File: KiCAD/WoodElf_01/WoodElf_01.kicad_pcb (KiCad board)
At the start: 2 copper layers, 97.7 x 102.4 mm, 122 parts, among them T10 BlankThrough-Hole, T11 BlankThrough-Hole, T12 BlankThrough-Hole, T13 BlankThrough-Hole, T2 BlankThrough-Hole, T3 BlankThrough-Hole, T4 BlankThrough-Hole, T5 BlankThrough-Hole, T6 BlankThrough-Hole, T7 BlankThrough-Hole, T8 BlankThrough-Hole, T9 BlankThrough-Hole

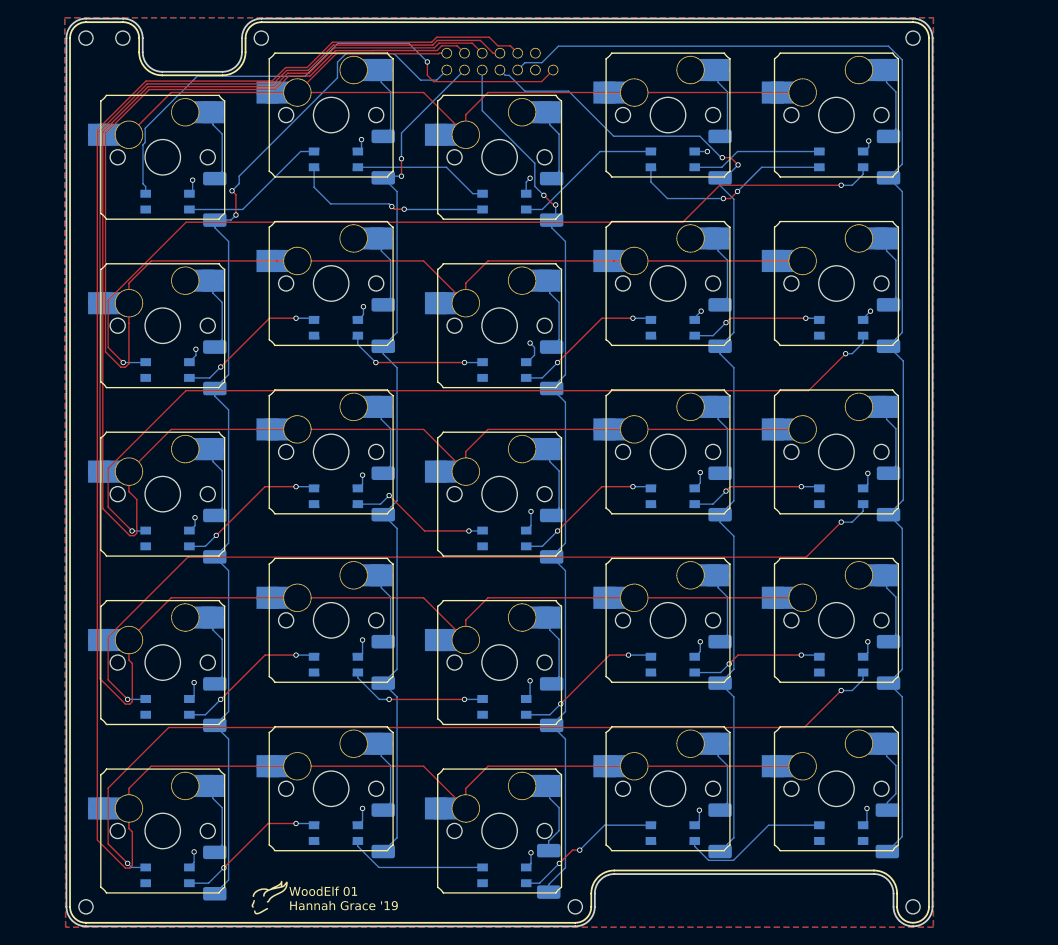
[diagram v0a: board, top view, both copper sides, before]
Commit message: completely redid everything
properly this time.
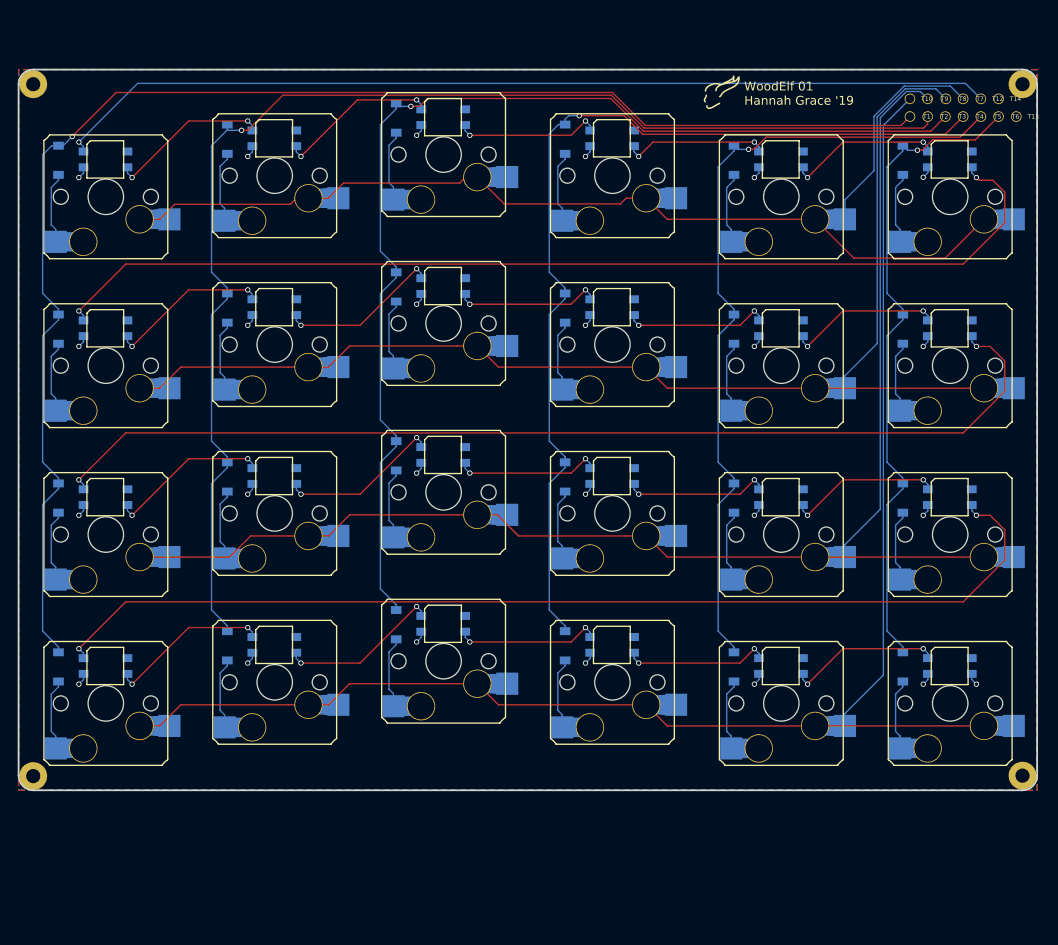
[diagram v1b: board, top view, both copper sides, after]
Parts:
- removed D21, D22, D23, D24, D25: DIODE, Diode_SMD:D_2010_5025Metric_Pad1.52x2.65mm_HandSolder
- removed the G*** at (135.0, 151.5)
- removed the G*** at (121.0, 151.6)
- removed H21, H22, H23, H24, H25: Kailh_HotSwap_SwitchMount, WoodElf_Lib:Kailh_HotSwap_Socket
- removed L21, L22, L23, L24, L25: SK6812MINI, WoodElf_Lib:LED_SK6812MINI_PLCC4_3.5x3.5mm_P1.75mm
- removed the Mount at (120.1, 54.4)
- removed the Mount at (104.5, 54.4)
- removed the Mount at (155.5, 152.4)
- removed the Mount at (193.6, 152.4)
- removed the Mount at (100.3, 152.4)
- removed the Mount at (100.3, 54.4)
- removed the Mount at (193.6, 54.4)
- removed S21, S22, S23, S24, S25: Kailh_RGB_Switch, WoodElf_Lib:SW_Cherry_MX1A_1.00u_PCB
- removed T11, wT1: BlankThrough-Hole, WoodElf_Lib:BlankThrough-Hole
- added D27: DIODE, WoodElf_Lib:D_SOD-123, B.Cu at (192.4, 125.3)
- added D28: DIODE, WoodElf_Lib:D_SOD-123, B.Cu at (192.4, 106.3)
- added D29: DIODE, WoodElf_Lib:D_SOD-123, B.Cu at (192.4, 87.2)
- added D30: DIODE, WoodElf_Lib:D_SOD-123, B.Cu at (192.4, 68.2)
- added G***: Tiefling_Logo, WoodElf_Lib:Tiefling_Logo, B.Cu at (186.3, 60.8)
- added G***: Tiefling_Logo, WoodElf_Lib:Tiefling_Logo, F.Cu at (172.0, 60.8)
- added H27: Kailh_HotSwap_SwitchMount, WoodElf_Lib:Kailh_HotSwap_Socket, F.Cu at (195.2, 134.5)
- added H28: Kailh_HotSwap_SwitchMount, WoodElf_Lib:Kailh_HotSwap_Socket, F.Cu at (195.2, 115.5)
- added H29: Kailh_HotSwap_SwitchMount, WoodElf_Lib:Kailh_HotSwap_Socket, F.Cu at (195.2, 96.4)
- added H30: Kailh_HotSwap_SwitchMount, WoodElf_Lib:Kailh_HotSwap_Socket, F.Cu at (195.2, 77.4)
- added L27: SK6812MINI, WoodElf_Lib:LED_SK6812MINI_PLCC4_3.5x3.5mm_P1.75mm, F.Cu at (197.8, 125.2)
- added L28: SK6812MINI, WoodElf_Lib:LED_SK6812MINI_PLCC4_3.5x3.5mm_P1.75mm, F.Cu at (197.8, 106.2)
- added L29: SK6812MINI, WoodElf_Lib:LED_SK6812MINI_PLCC4_3.5x3.5mm_P1.75mm, F.Cu at (197.8, 87.1)
- added L30: SK6812MINI, WoodElf_Lib:LED_SK6812MINI_PLCC4_3.5x3.5mm_P1.75mm, F.Cu at (197.8, 68.1)
- added Mount: Mount, WoodElf_Lib:Mount, F.Cu at (94.3, 59.6)
- added Mount: Mount, WoodElf_Lib:Mount, F.Cu at (94.3, 137.7)
- added Mount: Mount, WoodElf_Lib:Mount, F.Cu at (205.9, 137.6)
- added Mount: Mount, WoodElf_Lib:Mount, F.Cu at (205.9, 59.6)
- added S27: Kailh_RGB_Switch, WoodElf_Lib:SW_Cherry_MX1A_1.00u_PCB, F.Cu at (195.2, 134.5)
- added S28: Kailh_RGB_Switch, WoodElf_Lib:SW_Cherry_MX1A_1.00u_PCB, F.Cu at (195.2, 115.5)
- added S29: Kailh_RGB_Switch, WoodElf_Lib:SW_Cherry_MX1A_1.00u_PCB, F.Cu at (195.2, 96.4)
- added S30: Kailh_RGB_Switch, WoodElf_Lib:SW_Cherry_MX1A_1.00u_PCB, F.Cu at (195.2, 77.4)
- added T1: BlankThrough-Hole, WoodElf_Lib:BlankThrough-Hole, F.Cu at (193.2, 63.2)
- added T14: BlankThrough-Hole, WoodElf_Lib:BlankThrough-Hole, F.Cu at (203.2, 61.2)
- D1, D10, D11, D12, D13, D14, D15, D16, D17, D18, D19, D2, D20, D3, D4, D5, D6, D7, D8, D9: footprint Diode_SMD:D_2010_5025Metric_Pad1.52x2.65mm_HandSolder -> WoodElf_Lib:D_SOD-123
- moved T6 62.7 mm to (203.2, 63.2)
- moved T7 56.5 mm to (199.2, 61.2)
- moved T13 54.5 mm to (205.2, 63.2)
- moved T8 52.6 mm to (197.3, 61.2)
- moved T2 52.5 mm to (195.2, 63.2)
- moved T3 52.5 mm to (197.2, 63.2)
- moved T4 52.5 mm to (199.2, 63.2)
- moved T5 52.5 mm to (201.2, 63.2)
- moved T12 50.5 mm to (201.2, 61.2)
- moved T9 48.5 mm to (195.2, 61.2)
- moved T10 44.5 mm to (193.2, 61.2)
- moved H16 22.6 mm to (176.2, 134.5), turned to 180 degrees
- moved S16 22.6 mm to (176.2, 134.5), turned to 180 degrees
- moved H15 22.5 mm to (176.2, 115.5), turned to 180 degrees
- moved S15 22.5 mm to (176.2, 115.5), turned to 180 degrees
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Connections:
- L15 pad 1: /sheet5D51F414/Din -> /sheet5D22F5C7/Din
- L16 pad 1: /sheet5D526D44/Din -> /sheet5D22F5C1/Din
- L5 pad 1: /sheet5D4D3834/Din -> /sheet5D22F5D3/Din
- L6 pad 1: /sheet5D4DB164/Din -> /sheet5D22F5CD/Din
- T10 pad 1: /Row5 -> /Row4
- T12 pad 1: VDD -> /Din
- T13 pad 1: VSS -> VDD
- T6 pad 1: /Row1 -> /Col6
- T7 pad 1: /Row2 -> /Row1
- T8 pad 1: /Row3 -> /Row2
- T9 pad 1: /Row4 -> /Row3
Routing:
- net /Row5: track 246.0 -> 0.00 mm
- net /sheet5D526D44/Din: track 102.7 -> 0.00 mm, vias 2 -> 0
- net /Col6: track 0.00 -> 74.2 mm, vias 0 -> 1
- net /Col5: track 140.4 -> 91.2 mm, vias 0 -> 1
- net VDD: track 47.7 -> 0.00 mm, vias 25 -> 0
- net /Col2: track 98.2 -> 144.8 mm, vias 2 -> 1
- net /Din: track 60.8 -> 106.5 mm
- net /Col1: track 120.5 -> 162.5 mm, vias 2 -> 1
- net /Row4: track 223.9 -> 193.2 mm
- net /Row1: track 118.8 -> 148.6 mm
- net /Row3: track 202.5 -> 177.5 mm
- net /Col3: track 101.8 -> 126.3 mm, vias 2 -> 1
- net /Row2: track 181.3 -> 161.0 mm
- net /sheet5D22F5C1/Din: track 0.00 -> 17.4 mm, vias 0 -> 2
- net /sheet5D22F5D3/Din: track 0.00 -> 17.4 mm, vias 0 -> 2
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- added copper zone on B.Cu, net VDD
- added copper zone on F.Cu, net VSS
- removed copper zone on F.Cu, net VDD
- removed copper zone on B.Cu, net VSS
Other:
- board size 97.7 x 102.4 mm -> 114.9 x 81.3 mm
- board text removed: "C1"
- board text removed: "C2"
- board text removed: "C3"
- board text removed: "C4"
- board text removed: "C5"
- board text removed: "Din"
- board text removed: "R1"
- board text removed: "R2"
- board text removed: "R3"
- board text removed: "R4"
- board text removed: "R5"
- board text removed: "VDD"
- board text removed: "VSS"
